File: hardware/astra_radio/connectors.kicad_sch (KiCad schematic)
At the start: 2 parts, among them J1 SM04B-GHS-TB

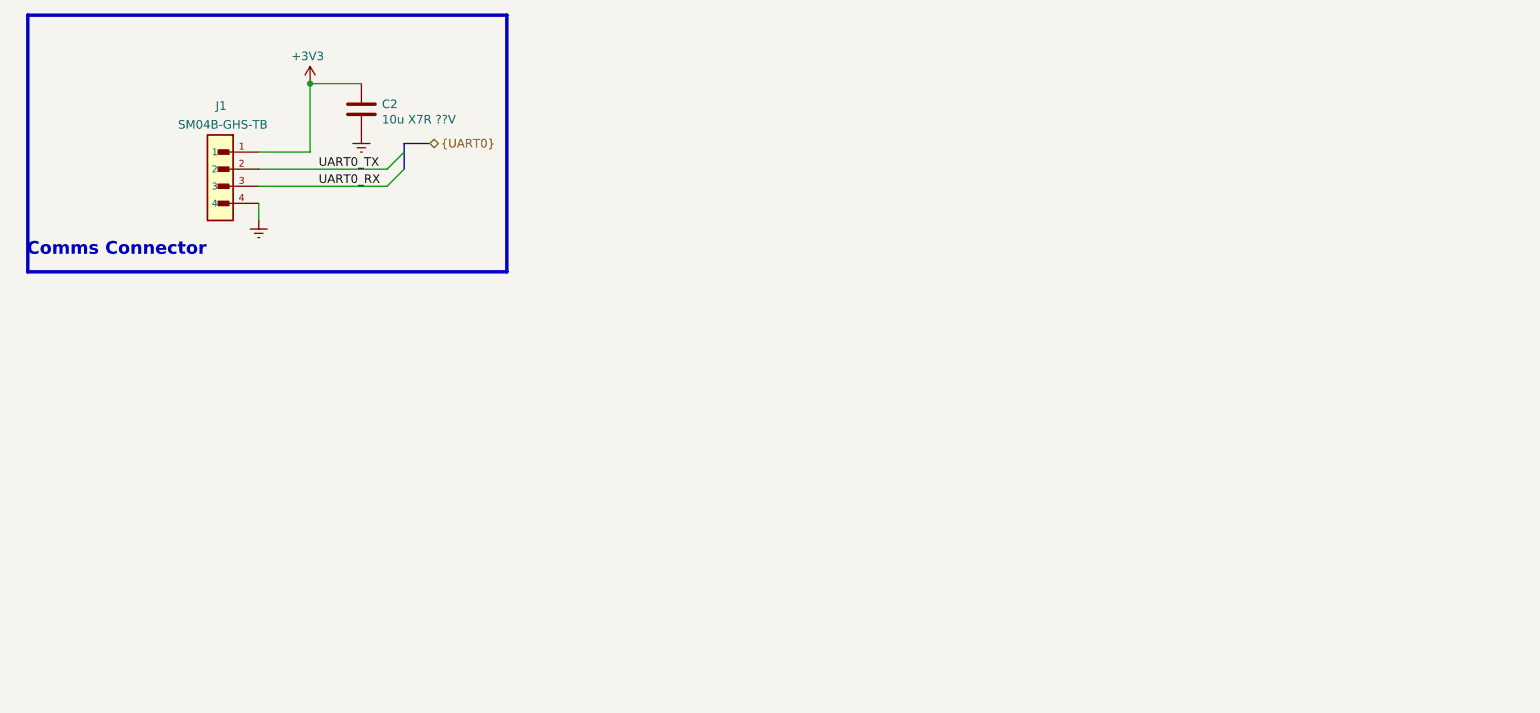
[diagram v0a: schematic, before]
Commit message: Lots of new stuff, but lost some stuff :-)
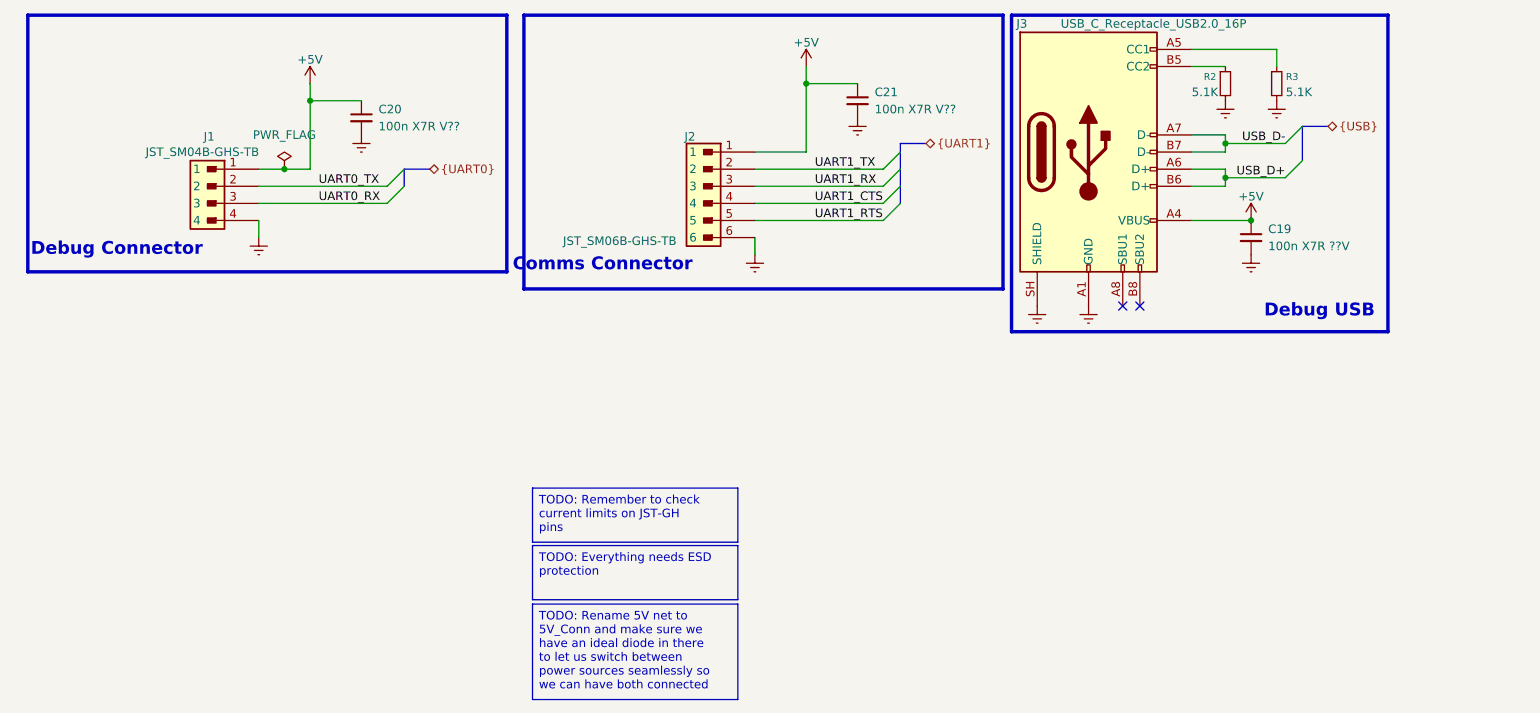
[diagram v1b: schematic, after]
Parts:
- removed C2: 10u X7R ??V, Capacitor_SMD:C_0603_1608Metric, symbol Device:C
- added C19: 100n X7R ??V, symbol Device:C_Small
- added C20, C21: 100n X7R V??, symbol Device:C_Small
- added J2: JST_SM06B-GHS-TB, astra_parts:JST_SM06B-GHS-TB, symbol astra_parts:JST_SM06B-GHS-TB
- added J3: USB_C_Receptacle_USB2.0_16P, symbol astra_parts:USB_C_Receptacle_USB2.0_16P
- added R2, R3: 5.1K, symbol Device:R_Small
- J1: value SM04B-GHS-TB -> JST_SM04B-GHS-TB; footprint SM04B-GHS-TB:JST_SM04B-GHS-TB -> astra_parts:JST_SM04B-GHS-TB; symbol astra_parts:SM04B-GHS-TB -> astra_parts:JST_SM04B-GHS-TB; MANUFACTURER JST -> (none)
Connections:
- net Earth: now also C19.2, C20.2, C21.2, J2.6, J3.A1 (GND), J3.A12 (GND), J3.B1 (GND), J3.B12 (GND), J3.SH (SHIELD), R2.2, R3.2
- net +3V3 renamed +5V
- net +5V: now also C19.1, C20.1, C21.1, J2.1, J3.A4 (VBUS), J3.A9 (VBUS), J3.B4 (VBUS), J3.B9 (VBUS)
- new net: J3.A5 (CC1), R3.1
- new net: J3.B5 (CC2), R2.1
- new net UART1_CTS: J2.4
- new net UART1_RTS: J2.5
- new net UART1_RX: J2.3
- new net UART1_TX: J2.2
- new net USB_D+: J3.A6 (D+), J3.B6 (D+)
- new net USB_D-: J3.A7 (D-), J3.B7 (D-)
- no-connect marks 0 -> 2
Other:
- note added: "Debug Connector"
- note added: "Debug USB"
- moved on the sheet: J1

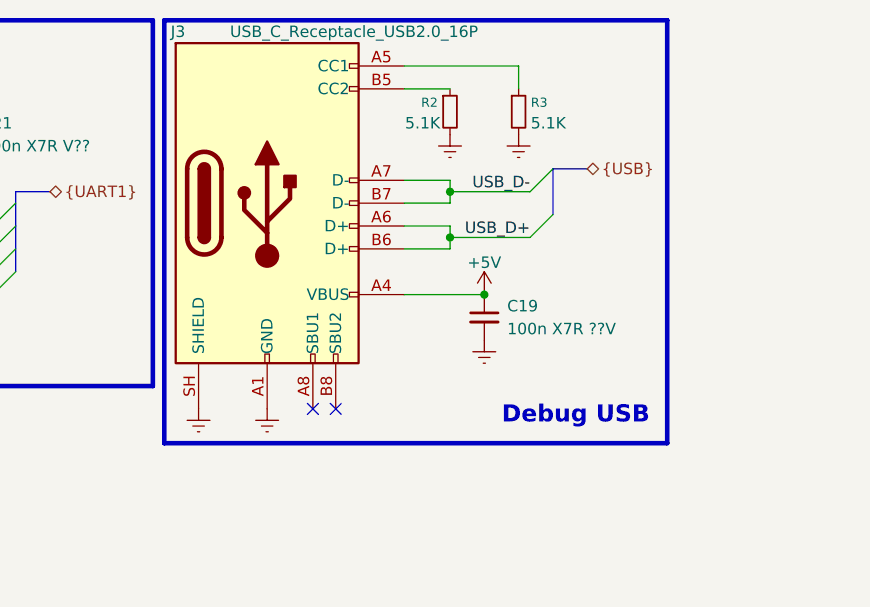
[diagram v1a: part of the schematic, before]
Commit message: Alsmot there
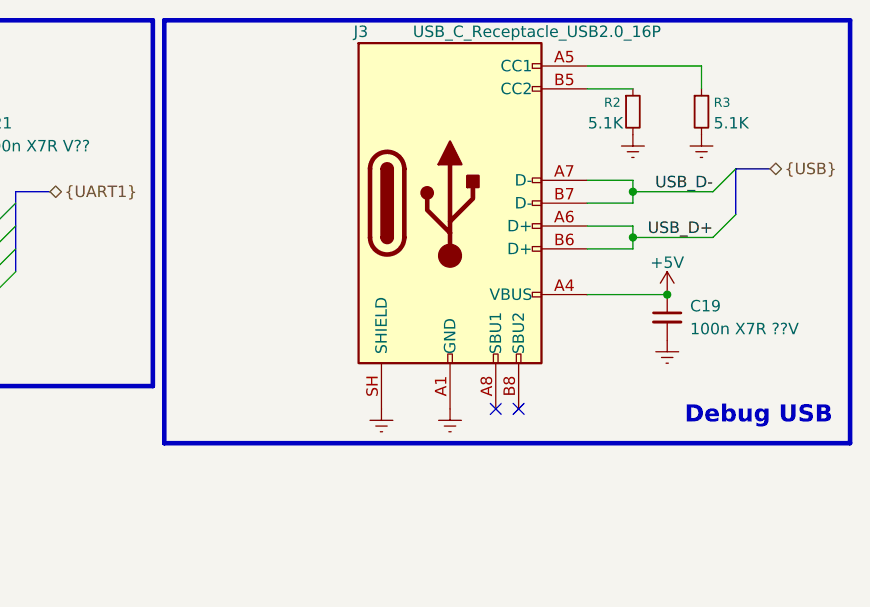
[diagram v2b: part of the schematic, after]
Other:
- moved on the sheet: C19, J3, R2, R3
